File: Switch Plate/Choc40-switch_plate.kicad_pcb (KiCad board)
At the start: 2 copper layers, 216 x 70.8 mm, 100 parts, among them SW1 SW_Push, SW10 SW_Push, SW11 SW_Push, SW12 SW_Push, SW13 SW_Push, SW14 SW_Push, SW15 SW_Push, SW16 SW_Push, SW17 SW_Push, SW18 SW_Push, SW19 SW_Push, SW2 SW_Push, SW20 SW_Push, SW21 SW_Push, SW22 SW_Push, SW23 SW_Push, SW24 SW_Push, SW25 SW_Push, SW26 SW_Push, SW27 SW_Push, SW28 SW_Push, SW29 SW_Push, SW3 SW_Push, SW30 SW_Push, SW31 SW_Push, SW32 SW_Push, SW33a1 SW_Push, SW33b1 SW_Push, SW34a1 SW_Push, SW34b1 SW_Push, SW35 SW_Push, SW36 SW_Push, SW37 SW_Push, SW38 SW_Push, SW39 SW_Push, SW4 SW_Push, SW40 SW_Push, SW5 SW_Push, SW6 SW_Push, SW7 SW_Push, SW8 SW_Push, SW9 SW_Push, SW99 SW_Push, U1 ATmega32U2-MU, Y1 Resonator_Small

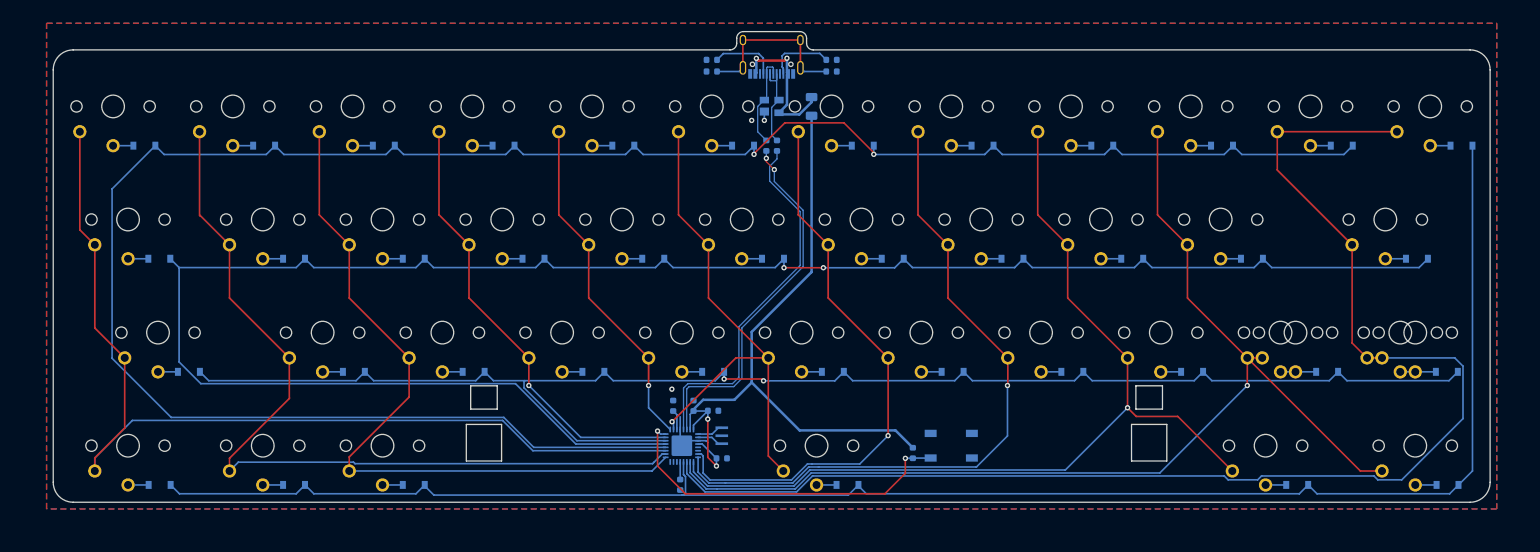
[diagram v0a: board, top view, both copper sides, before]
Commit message: Production files added
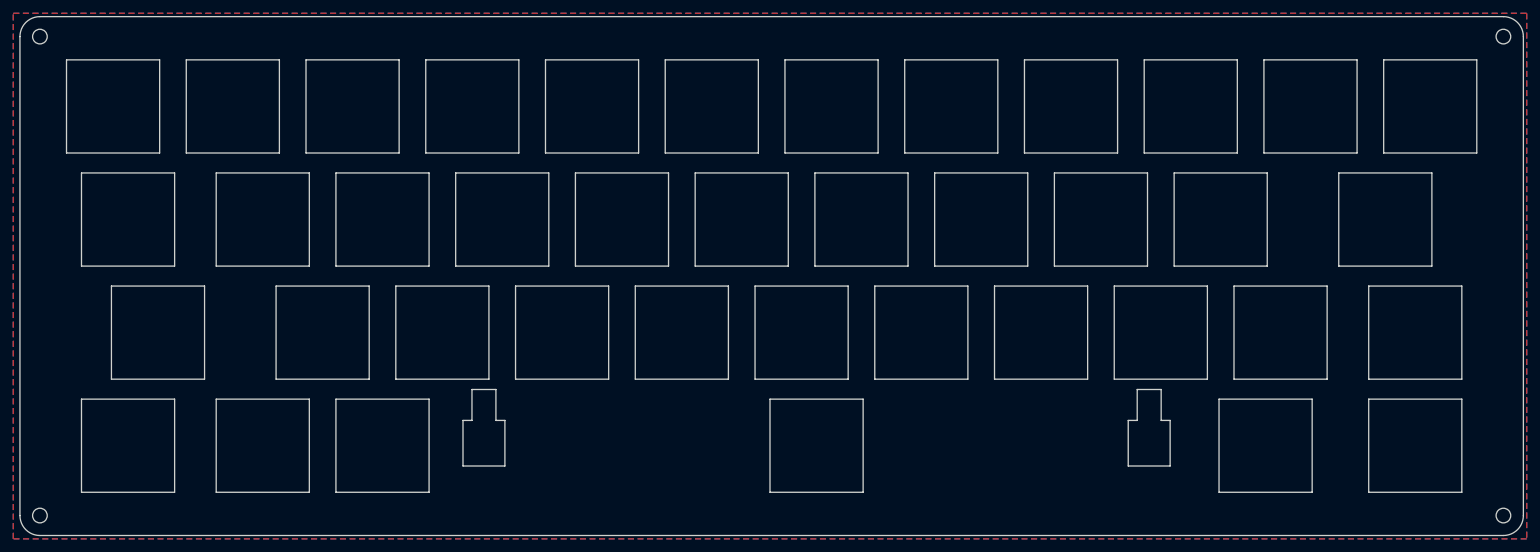
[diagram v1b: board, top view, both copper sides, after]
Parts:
- removed C1: 1uF, Capacitor_SMD:C_0603_1608Metric
- removed C2, C3: 0.1uF, Capacitor_SMD:C_0603_1608Metric
- removed C4: 10uF, Capacitor_SMD:C_0603_1608Metric
- removed C5: 4.7n, Capacitor_SMD:C_0603_1608Metric
- removed D1, D10, D11, D12, D13, D14, D15, D16, D17, D18, D19, D2, D20, D21, D22, D23, D24, D25, D26, D27, D28, D29, D3, D30, D31, D32, D33, D34, D35, D36, D37, D38, D39, D4, D40, D5, D6, D7, D8, D9: D_Small, Diode_SMD:D_SOD-123
- removed D41: PRTR5V0U2X, Package_TO_SOT_SMD:SOT-143
- removed F1: 500mA, Fuse:Fuse_1206_3216Metric
- removed R1, R4: 10k, Resistor_SMD:R_0603_1608Metric
- removed R2, R3: 22, Resistor_SMD:R_0603_1608Metric
- removed R5, R6: 5k1, Resistor_SMD:R_0603_1608Metric
- removed R7: 1M, Resistor_SMD:R_0603_1608Metric
- removed SW33b1: SW_Push, mbk:Choc-1.25u-solder
- removed SW34b1: SW_Push, mbk:Choc-1u-solder
- removed SW99: SW_Push, random-keyboard-parts:SKQG-1155865
- removed U1: ATmega32U2-MU, Package_DFN_QFN:QFN-32-1EP_5x5mm_P0.5mm_EP3.1x3.1mm
- removed USB1: HRO-TYPE-C-31-M-12, Type-C:HRO-TYPE-C-31-M-12
- removed Y1: Resonator_Small, Crystal:Resonator_SMD_muRata_CSTxExxV-3Pin_3.0x1.1mm
- added H1: MountingHole, MountingHole:MountingHole_2.2mm_M2, F.Cu at (23.0, 23.0)
- added H2: MountingHole, MountingHole:MountingHole_2.2mm_M2, F.Cu at (23.0, 95.0)
- added H3: MountingHole, MountingHole:MountingHole_2.2mm_M2, F.Cu at (243.0, 23.0)
- added H4: MountingHole, MountingHole:MountingHole_2.2mm_M2, F.Cu at (243.0, 95.0)
- SW1, SW10, SW11, SW12, SW14, SW15, SW16, SW17, SW18, SW19, SW2, SW20, SW21, SW22, SW25, SW26, SW27, SW28, SW29, SW3, SW30, SW31, SW32, SW33a1, SW36, SW37, SW4, SW5, SW6, SW7, SW8, SW9: footprint mbk:Choc-1u-solder -> mbk:Choc-1u-cutout
- SW13, SW34a1, SW35, SW39, SW40: footprint mbk:Choc-1.25u-solder -> mbk:Choc-1u-cutout
- SW23, SW24: footprint mbk:Choc-1.75u-solder -> mbk:Choc-1u-cutout
- SW38: footprint mbk:Choc-6.25u-solder -> mbk:Choc-6.25u-cutout
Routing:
- net row0: track 319.5 -> 0.00 mm, vias 2 -> 0
- net row1: track 293.3 -> 0.00 mm, vias 2 -> 0
- net row3: track 256.7 -> 0.00 mm
- net row2: track 226.4 -> 0.00 mm, vias 2 -> 0
- net col10: track 205.5 -> 0.00 mm
- net col9: track 166.1 -> 0.00 mm, vias 1 -> 0
- net col0: track 147.6 -> 0.00 mm
- net col8: track 139.3 -> 0.00 mm, vias 1 -> 0
- net col1: track 127.7 -> 0.00 mm
- net col2: track 108.7 -> 0.00 mm
- net +5V: track 105.3 -> 0.00 mm, vias 2 -> 0
- net col7: track 103.7 -> 0.00 mm, vias 1 -> 0
- net col6: track 85.7 -> 0.00 mm, vias 1 -> 0
- net col5: track 77.2 -> 0.00 mm, vias 1 -> 0
- net col3: track 67.5 -> 0.00 mm, vias 1 -> 0
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- added copper zone on B.Cu, net (none)
- added copper zone on F.Cu, net (none)
- removed copper zone on B.Cu, net GND
- removed copper zone on F.Cu, net GND
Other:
- board size 216 x 70.8 mm -> 226 x 78 mm
